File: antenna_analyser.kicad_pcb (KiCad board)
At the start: 2 copper layers, 100 x 50 mm, 34 parts, among them IC1 MCP6002, IC2 ARDUINO_PRO_MINI_3.3V, P1 AD9850_CONN, P2 BNC, P3 CONN_LCD, P4 USB_OTG, P5 CONN_PROG, U1 AMS1117

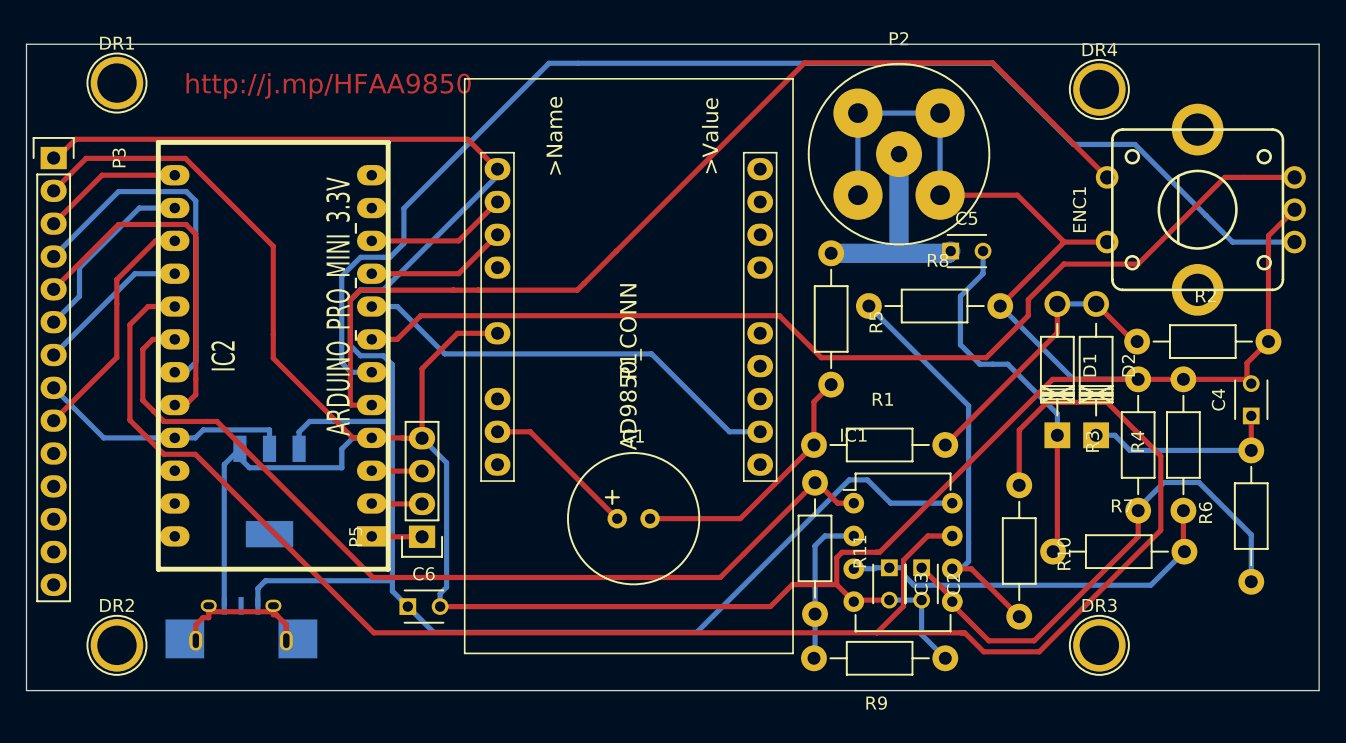
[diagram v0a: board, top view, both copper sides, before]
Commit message: Production artifacts.
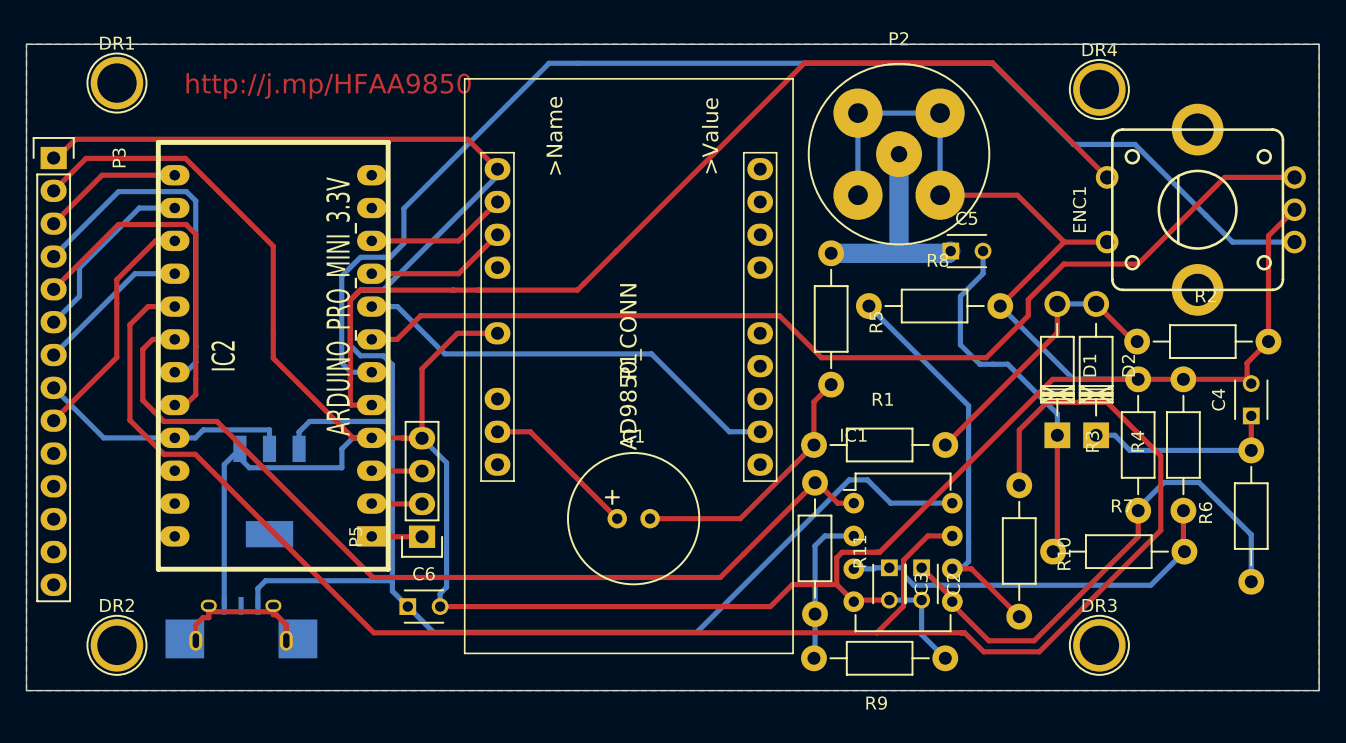
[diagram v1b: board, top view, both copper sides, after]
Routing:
- added copper zone on B.Cu, net GND
- added copper zone on F.Cu, net GND
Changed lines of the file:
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@@
-(kicad_pcb (version 4) (host pcbnew "(2015-06-03 BZR 5697)-product")
+(kicad_pcb (version 4) (host pcbnew 4.0.6)
   (general
     (links 72)
     (no_connects 0)
-    (area 70.714287 64.15 223 159.700001)
+    (area 70.864287 64.3 222.85 159.700001)
     (thickness 1.6)
     (drawings 9)
@@
     (pad_to_mask_clearance 0)
     (aux_axis_origin 0 0)
-    (visible_elements FFFFFF7F)
+    (visible_elements FFFFEF7F)
     (pcbplotparams
-      (layerselection 0x00000_80000000)
+      (layerselection 0x3ffff_80000001)
       (usegerberextensions false)
       (excludeedgelayer true)
@@
       (padsonsilk false)
       (subtractmaskfromsilk false)
-      (outputformat 4)
+      (outputformat 1)
       (mirror false)
-      (drillshape 2)
+      (drillshape 0)
       (scaleselection 1)
-      (outputdirectory production/))
+      (outputdirectory gerber))
   )
   (net 0 "")
@@
   (segment (start 109.3201 128.1314) (end 110.1009 128.9122) (width 0.4) (layer F.Cu) (net 53))
   (segment (start 109.1009 128.1314) (end 109.3201 128.1314) (width 0.4) (layer F.Cu) (net 53))
+  (zone (net 5) (net_name GND) (layer F.Cu) (hatch edge 0.508)
+    (connect_pads (clearance 0.508))
+    (min_thickness 0.254)
+    (fill yes (arc_segments 16) (thermal_gap 0.508) (thermal_bridge_width 0.508))
+    (polygon
+      (pts
+        (xy 90 84) (xy 190 84) (xy 190 134) (xy 90 134)
+      )
+    )
+  )
+  (zone (net 5) (net_name GND) (layer B.Cu) (hatch edge 0.508)
+    (connect_pads (clearance 0.508))
+    (min_thickness 0.254)
+    (fill yes (arc_segments 16) (thermal_gap 0.508) (thermal_bridge_width 0.508))
+    (polygon
+      (pts
+        (xy 90 84) (xy 190 84) (xy 190 134) (xy 90 134)
+      )
+    )
+  )
 )
